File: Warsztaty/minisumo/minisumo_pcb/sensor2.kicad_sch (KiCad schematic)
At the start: 1 part

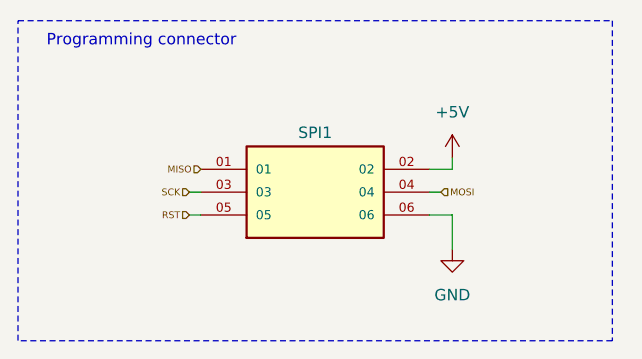
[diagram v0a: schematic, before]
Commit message: chyba gotowy schemat
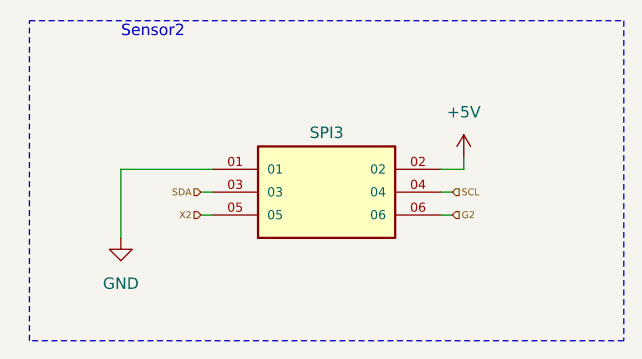
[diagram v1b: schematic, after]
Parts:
- removed SPI1: MTSW-103-23-F-D-230, MTSW-103-23-F-D-230:SAMTEC_MTSW-103-23-F-D-230, symbol MTSW-103-23-F-D-230:MTSW-103-23-F-D-230
- added SPI3: MTSW-103-23-F-D-230, MTSW-103-23-F-D-230:SAMTEC_MTSW-103-23-F-D-230, symbol MTSW-103-23-F-D-230:MTSW-103-23-F-D-230
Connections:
- net +5V: now also SPI3.02
- net GND: now also SPI3.01
- new net G2: SPI3.06
- new net SCL: SPI3.04
- new net SDA: SPI3.03
- new net X2: SPI3.05
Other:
- note added: "Sensor2"
- note removed: "Programming connector"
